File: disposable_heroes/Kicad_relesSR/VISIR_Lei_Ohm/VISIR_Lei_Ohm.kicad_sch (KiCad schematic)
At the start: 4 parts, among them K1 3572-1220-053

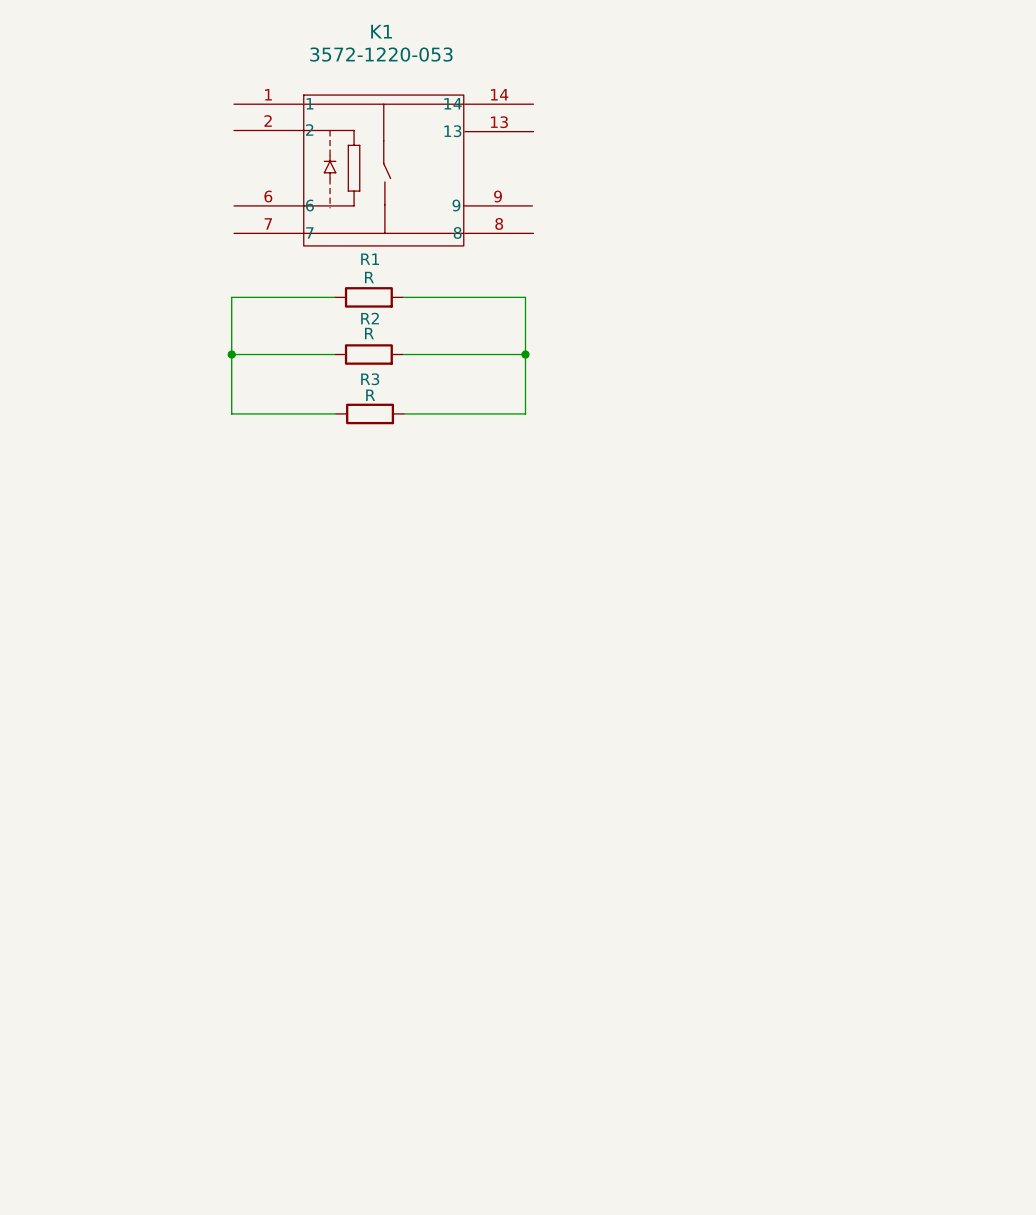
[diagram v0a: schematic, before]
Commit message: update kicad
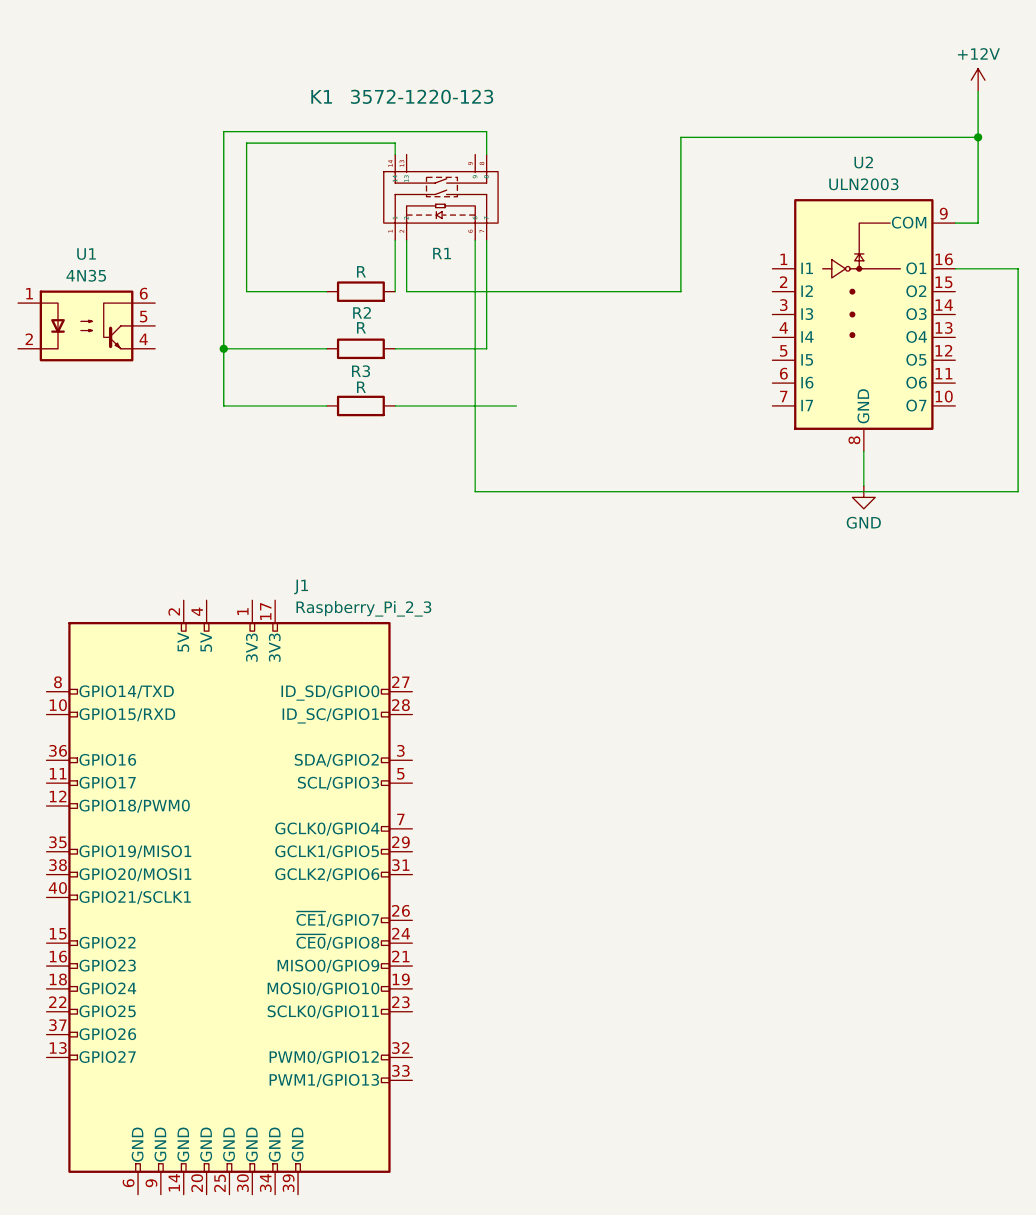
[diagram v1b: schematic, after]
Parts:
- removed K1: 3572-1220-053, RELAY8_3572-1220-053_COM, symbol rele_DPST_Tese:3572-1220-053
- added J1: Raspberry_Pi_2_3, symbol Connector:Raspberry_Pi_2_3
- added K1: 3572-1220-123, RELAY8_3572-1220-053_COM, symbol 3572-1220-123:3572-1220-123
- added U1: 4N35, Package_DIP:DIP-6_W7.62mm, symbol Isolator:4N35
- added U2: ULN2003, symbol Transistor_Array:ULN2003
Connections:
- net at R2.1, R3.1: now also K1.8; no longer R1.1
- new net: K1.14, R1.1
- new net: K1.1, R1.2
- new net: K1.6, U2.16 (O1)
- new net: K1.7, R2.2
- new net +12V: K1.2, U2.9 (COM)
- new net GND: U2.8 (GND)
- now unconnected: R3.2
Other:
- moved on the sheet: R1, R2, R3
